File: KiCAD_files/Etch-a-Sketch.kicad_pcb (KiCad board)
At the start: 2 copper layers, 98 x 85.5 mm, 45 parts, among them J1 Debug Connector, J2 Display / Mounting Socket, J3 Display Mounting Socket, P1 PHR-2, U1 STM32L433CCTx, U2 W25Q64JV, U3 ICM-42688-P, U6 Adafruit 377 Rotary Encoder, U7 Adafruit 377 Rotary Encoder

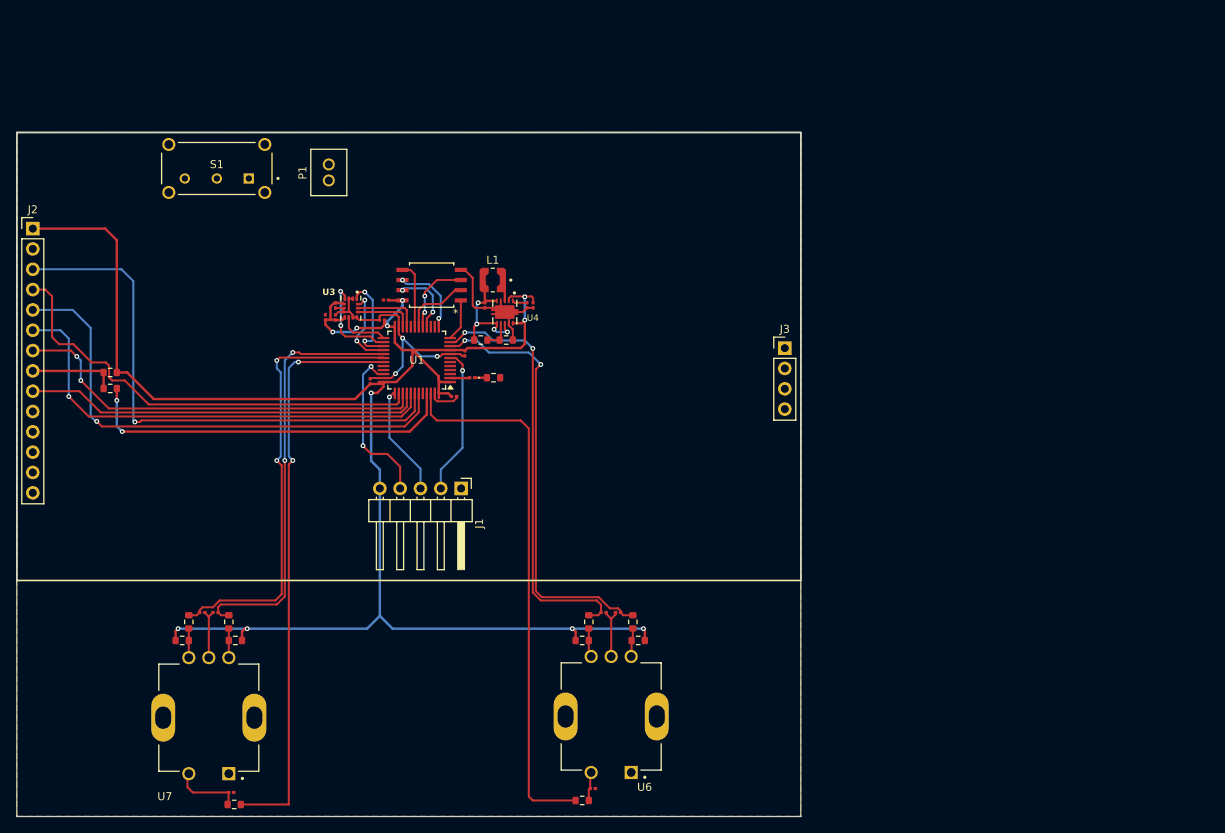
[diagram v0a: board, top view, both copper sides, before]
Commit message: PCB layout draft and clean files
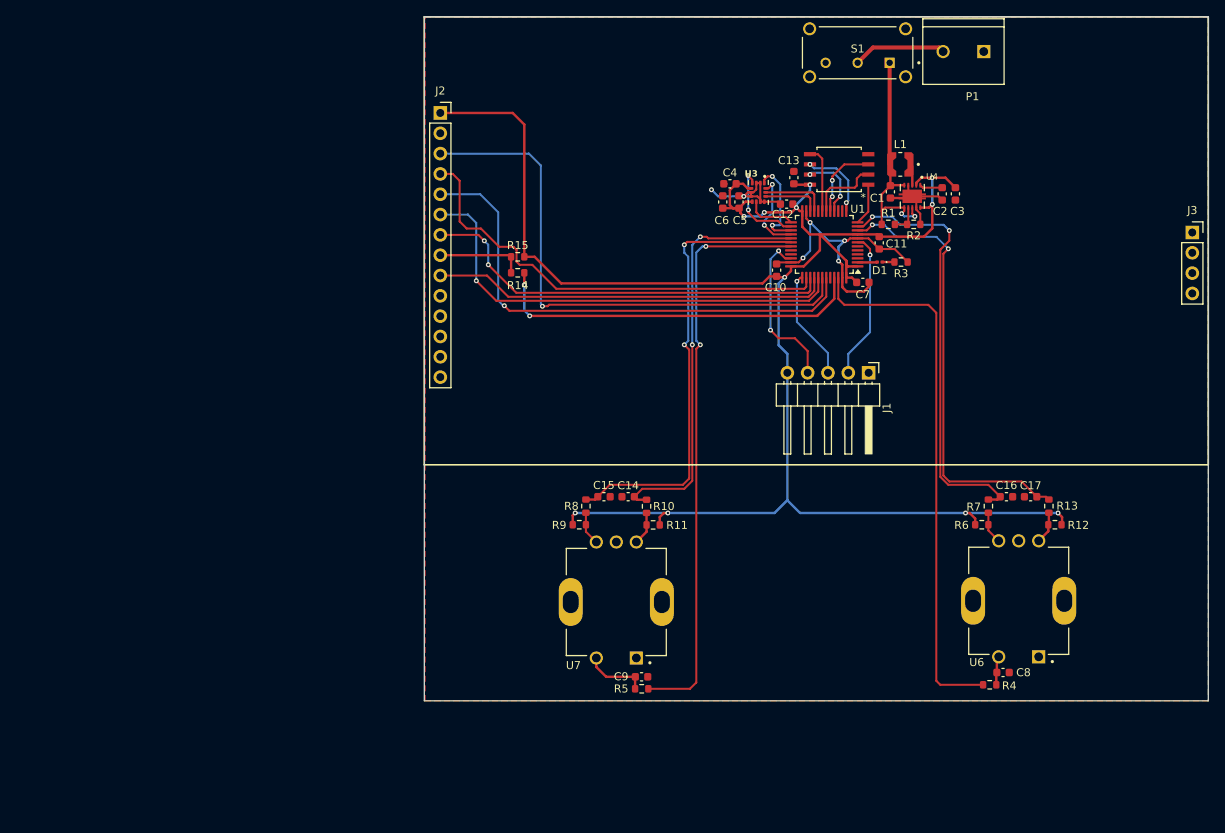
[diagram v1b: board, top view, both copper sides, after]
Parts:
- C1, C10, C11, C12, C13, C14, C15, C16, C17, C2, C3, C4, C5, C6, C7, C8, C9: footprint Capacitor_SMD:C_0201_0603Metric -> Capacitor_SMD:C_0603_1608Metric
- J2: footprint Connector_PinHeader_2.54mm:PinHeader_1x14_P2.54mm_Vertical -> Connector_PinSocket_2.54mm:PinSocket_1x14_P2.54mm_Vertical
- J3: footprint Connector_PinHeader_2.54mm:PinHeader_1x04_P2.54mm_Vertical -> Connector_PinSocket_2.54mm:PinSocket_1x04_P2.54mm_Vertical
- P1: value PHR-2 -> 282837-2; footprint PHR_2:JST_PHR-2 -> 282837_2:TE_282837-2
- moved S1 81.4 mm to (158.6, 56.5)
- moved P1 80.8 mm to (171.8, 56.4), turned to 180 degrees
- moved C3 54.6 mm to (170.8, 74.2)
- moved R11 54.2 mm to (133.0, 115.6)
- moved R10 54.2 mm to (132.2, 113.2)
- moved R12 54.1 mm to (183.3, 115.5)
- moved R13 54.0 mm to (182.5, 113.2)
- moved C2 53.7 mm to (169.2, 74.2)
- moved C11 53.6 mm to (161.3, 80.3)
- moved C14 53.6 mm to (129.9, 112.0)
- moved C17 53.6 mm to (180.2, 112.0)
- moved C9 53.3 mm to (131.6, 134.5)
- moved C8 53.3 mm to (176.8, 134.0)
- moved C13 53.2 mm to (150.6, 72.1), turned to 90 degrees
- moved C7 53.1 mm to (159.3, 85.2)
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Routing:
- net Net-(U4-EN): track 16.8 -> 29.8 mm, vias 4 -> 2
- net Net-(P1-Pad2): track 0.00 -> 11.7 mm
- net +3V3: track 231.2 -> 237.7 mm
- net GND: track 69.3 -> 63.8 mm, vias 3 -> 6
- net /QEI1_A: track 53.3 -> 52.0 mm
- net /QEI1_B: track 56.3 -> 57.4 mm
- net Net-(U4-VAUX): track 1.87 -> 2.87 mm
- net /QEI2_A: track 54.9 -> 55.9 mm
- net /QUADSPI_IO1: track 8.39 -> 9.08 mm
- net Net-(U7-Quad_B): track 3.65 -> 4.20 mm
- net Net-(U6-Quad_A): track 3.58 -> 4.11 mm
